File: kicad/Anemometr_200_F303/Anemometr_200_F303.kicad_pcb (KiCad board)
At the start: 2 copper layers, 25.8 x 45.3 mm, 44 parts, among them J1 Conn_01x01_Female, J10 USB_B_Micro, J11 Conn_01x01_Female, J12 Conn_01x01_Female, J13 Conn_01x01_Female, J14 Conn_01x01_Female, J15 Conn_01x01_Female, J16 Conn_01x01_Female, J17 Conn_01x01_Female, J18 Conn_01x01_Female, J19 Conn_01x01_Female, J2 Conn_01x01_Female, J20 Conn_01x01_Female, J21 Conn_01x01_Female, J22 Conn_01x01_Female, J23 Conn_01x01_Female, J24 Conn_01x01_Female, J25 Conn_01x01_Female, J26 Conn_01x01_Female, J27 Conn_01x01_Female, J3 Conn_01x01_Female, J4 Conn_01x01_Female, J5 Conn_01x01_Female, J6 Conn_01x01_Female, U1 AP1117-33, U2 STM32F303CCTx, U3 CH340C, Y1 16MHz

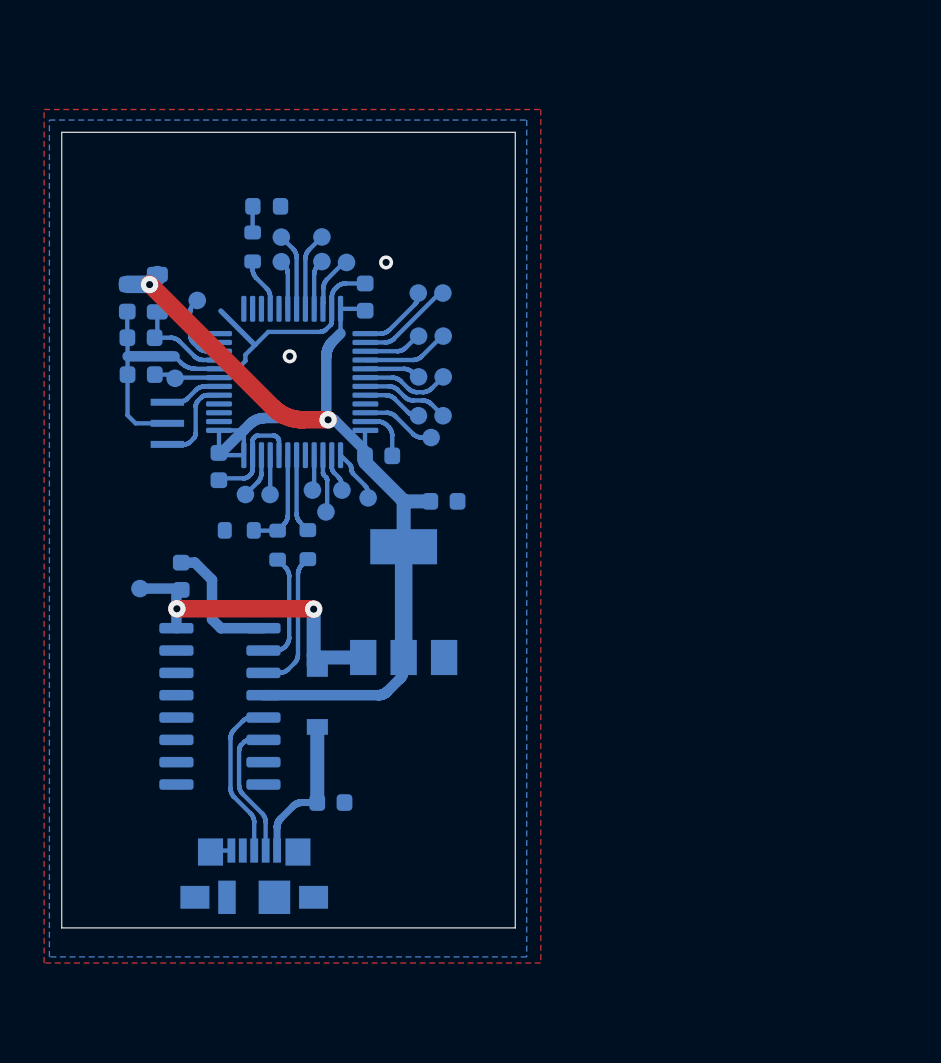
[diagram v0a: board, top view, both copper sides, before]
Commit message: изменено:      Documents/matLab/convData.m 	изменено:      kicad/Anemometr_200_F303/Anemometr_200_F303-cache.lib 	изменено:      kicad/Anemometr_200_F303/Anemometr_200_F303.kicad_pcb 	изменено:      kicad/Anemometr_200_F303/Anemometr_200_F303.kicad_pcb-bak 	изменено:      kicad/Anemometr_200_F303/Anemometr_200_F303.sch 	изменено:      kicad/Anemometr_200_F303/Anemometr_200_F303.sch-bak 	изменено:      kicad/Anemometr_200_F303/fp-info-cache 	изменено:      stm32cubeide/Anemometer_200_F303/Anemometer_200_F303.ioc 	новый файл:    stm32cubeide/Anemometer_200_F303/Core/Inc/FFTImplementationCallback.h 	изменено:      stm32cubeide/Anemometer_200_F303/Core/Inc/main.h 	новый файл:    stm32cubeide/Anemometer_200_F303/Core/Inc/maxEnvHilbert.h 	новый файл:    stm32cubeide/Anemometer_200_F303/Core/Inc/maxEnvHilbert_data.h 	новый файл:    stm32cubeide/Anemometer_200_F303/Core/Inc/maxEnvHilbert_terminate.h 	новый файл:    stm32cubeide/Anemometer_200_F303/Core/Inc/rt_nonfinite.h 	новый файл:    stm32cubeide/Anemometer_200_F303/Core/Inc/rtwtypes.h 	новый файл:    stm32cubeide/Anemometer_200_F303/Core/Inc/tmwtypes.h 	новый файл:    stm32cubeide/Anemometer_200_F303/Core/Src/FFTImplementationCallback.c 	изменено:      stm32cubeide/Anemometer_200_F303/Core/Src/main.c 	новый файл:    stm32cubeide/Anemometer_200_F303/Core/Src/maxEnvHilbert.c 	новый файл:    stm32cubeide/Anemometer_200_F303/Core/Src/maxEnvHilbert_data.c 	новый файл:    stm32cubeide/Anemometer_200_F303/Core/Src/maxEnvHilbert_terminate.c 	новый файл:    stm32cubeide/Anemometer_200_F303/Core/Src/rt_nonfinite.c 	изменено:      stm32cubeide/Anemometer_200_F303/Core/Src/stm32f3xx_hal_msp.c 	изменено:      stm32cubeide/Anemometer_200_F303/Core/Src/stm32f3xx_it.c 	изменено:      stm32cubeide/Anemometer_200_F303/Debug/Anemometer_200_F303.elf 	изменено:      stm32cubeide/Anemometer_200_F303/Debug/Anemometer_200_F303.list 	изменено:      stm32cubeide/Anemometer_200_F303/Debug/Anemometer_200_F303.map 	изменено:      stm32cubeide/Anemo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
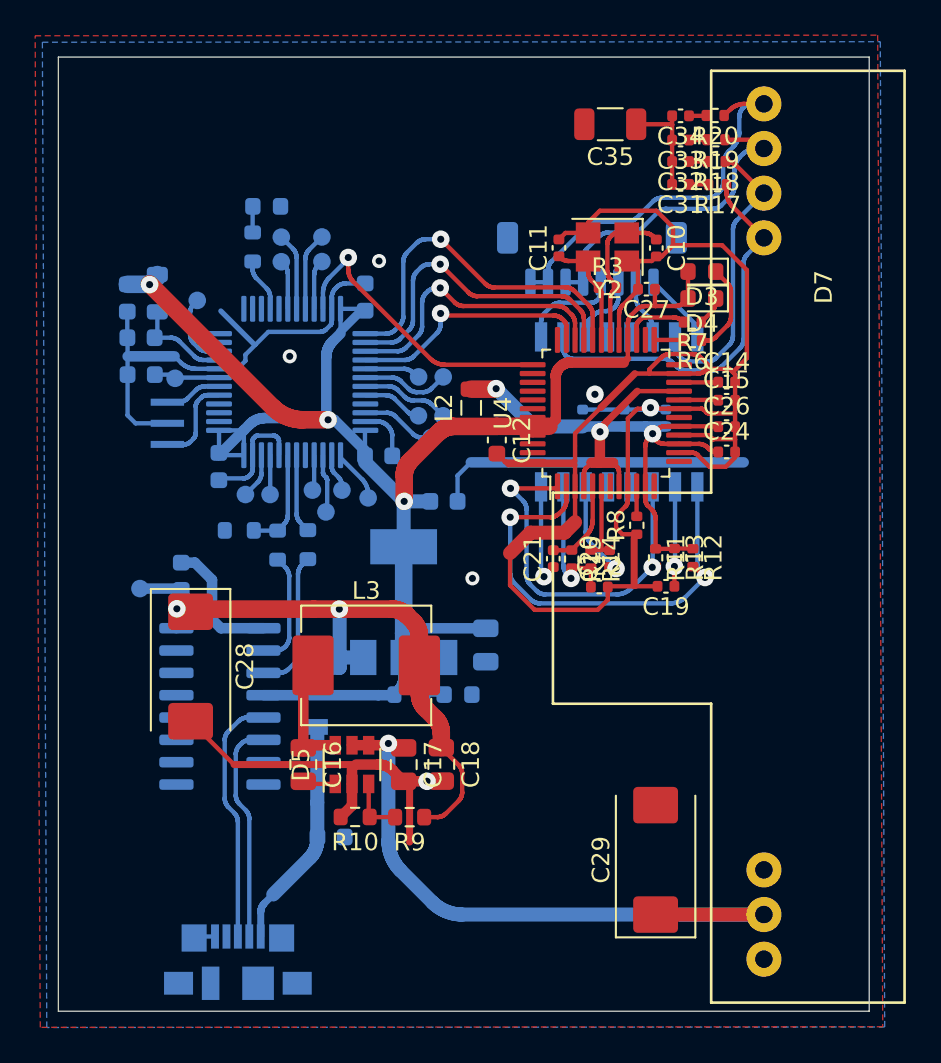
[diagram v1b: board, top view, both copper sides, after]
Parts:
- removed J18, J20, J21, J22, J24: Conn_01x01_Female, My-library:mini_conn
- added C10: C, Capacitor_SMD:C_0402_1005Metric, F.Cu at (65.3, 50.3)
- added C11: C, Capacitor_SMD:C_0402_1005Metric, F.Cu at (59.7, 50.3)
- added C12: C, Capacitor_SMD:C_0603_1608Metric, F.Cu at (56.2, 61.2)
- added C13: C, Capacitor_SMD:C_0402_1005Metric, B.Cu at (63.5, 60.0)
- added C14: 10n, Capacitor_SMD:C_0402_1005Metric, F.Cu at (69.3, 57.9)
- added C15: 4.7u, Capacitor_SMD:C_0402_1005Metric, F.Cu at (69.3, 59.0)
- added C16: 100n, Capacitor_SMD:C_0805_2012Metric, F.Cu at (45.2, 79.7)
- added C17: C, Capacitor_SMD:C_0805_2012Metric, F.Cu at (50.9, 79.7)
- added C18: C, Capacitor_SMD:C_0805_2012Metric, F.Cu at (53.0, 79.7)
- added C19: 22n, Capacitor_SMD:C_0402_1005Metric, F.Cu at (65.8, 69.5)
- added C20: 6.8n, Capacitor_SMD:C_0402_1005Metric, F.Cu at (62.6, 68.0)
- added C21: 6.8n, Capacitor_SMD:C_0402_1005Metric, F.Cu at (59.4, 68.0)
- added C22: 10n, Capacitor_SMD:C_0402_1005Metric, F.Cu at (62.0, 69.6)
- added C23: C, Capacitor_SMD:C_0402_1005Metric, B.Cu at (61.1, 60.0)
- added C24: C, Capacitor_SMD:C_0402_1005Metric, F.Cu at (69.3, 61.9)
- added C25: C, Capacitor_SMD:C_0402_1005Metric, B.Cu at (65.8, 60.0)
- added C26: C, Capacitor_SMD:C_0402_1005Metric, F.Cu at (69.3, 60.5)
- added C27: C, Capacitor_SMD:C_0402_1005Metric, F.Cu at (64.7, 52.6)
- added C28: 1000, Capacitor_Tantalum_SMD:CP_EIA-7343-15_Kemet-W, F.Cu at (38.8, 74.1)
- added C29: CP, Capacitor_Tantalum_SMD:CP_EIA-7343-15_Kemet-W, F.Cu at (65.2, 85.1)
- added C30: C, Capacitor_SMD:C_0805_2012Metric, B.Cu at (55.6, 72.9)
- added C31: 6.8n, Capacitor_SMD:C_0402_1005Metric, F.Cu at (66.7, 46.7)
- added C32: 6.8n, Capacitor_SMD:C_0402_1005Metric, F.Cu at (66.7, 45.4)
- added C33: 6.8n, Capacitor_SMD:C_0402_1005Metric, F.Cu at (66.7, 44.2)
- added C34: 6.8n, Capacitor_SMD:C_0402_1005Metric, F.Cu at (66.7, 42.8)
- added C35: 6.8n, Capacitor_SMD:C_1206_3216Metric, F.Cu at (62.7, 43.3)
- added D3: LED, LED_SMD:LED_0603_1608Metric, F.Cu at (67.9, 51.6)
- added D4: LED, LED_SMD:LED_0603_1608Metric, F.Cu at (67.9, 53.2)
- added D5: LMR50410, Package_TO_SOT_SMD:SOT-23-6, F.Cu at (48.0, 79.7)
- added D6: H1102NL, My-library:H1102N, B.Cu at (63.2, 59.6)
- added D7: RT9400, My-library:TR9400, F.Cu at (71.4, 52.2)
- added D8: LED, LED_SMD:LED_0603_1608Metric, B.Cu at (54.0, 75.7)
- added J7: Conn_01x08, Connector_JST:JST_SH_BM08B-SRSS-TB_1x08-1MP_P1.00mm_Vertical, B.Cu at (61.6, 50.9)
- added L2: L, Inductor_SMD:L_0805_2012Metric, F.Cu at (54.8, 59.4)
- added L3: 4.7u, Inductor_SMD:L_Abracon_ASPI-0630LR, F.Cu at (48.8, 74.0)
- added R10: 22.1k, Resistor_SMD:R_0603_1608Metric, F.Cu at (48.1, 82.7)
- added R11: 49R9, Resistor_SMD:R_0402_1005Metric, F.Cu at (65.2, 67.9)
- added R12: 49R9, Resistor_SMD:R_0402_1005Metric, F.Cu at (67.4, 67.9)
- added R13: 10R, Resistor_SMD:R_0402_1005Metric, F.Cu at (66.3, 67.9)
- added R14: 82R, Resistor_SMD:R_0402_1005Metric, F.Cu at (61.6, 68.0)
- added R15: 82R, Resistor_SMD:R_0402_1005Metric, F.Cu at (60.5, 68.0)
- added R16: 1k, Resistor_SMD:R_0603_1608Metric, B.Cu at (51.2, 75.7)
- added R17: 75, Resistor_SMD:R_0402_1005Metric, F.Cu at (68.8, 46.7)
- added R18: 75, Resistor_SMD:R_0402_1005Metric, F.Cu at (68.7, 45.4)
- added R19: 75, Resistor_SMD:R_0402_1005Metric, F.Cu at (68.7, 44.1)
- added R20: 75, Resistor_SMD:R_0402_1005Metric, F.Cu at (68.6, 42.8)
- added R3: 1M, Resistor_SMD:R_0402_1005Metric, F.Cu at (62.5, 52.5)
- added R6: 1M, Resistor_SMD:R_0402_1005Metric, F.Cu at (67.3, 55.6)
- added R7: 1M, Resistor_SMD:R_0402_1005Metric, F.Cu at (67.3, 54.5)
- added R8: 12.4k, Resistor_SMD:R_0402_1005Metric, F.Cu at (64.2, 66.1)
- added R9: 88.7k, Resistor_SMD:R_0603_1608Metric, F.Cu at (51.2, 82.7)
- added U4: W5500, Package_QFP:LQFP-48_7x7mm_P0.5mm, F.Cu at (62.4, 59.7)
- added Y2: Crystal_GND24_Small, Crystal:Crystal_SMD_SeikoEpson_FA238-4Pin_3.2x2.5mm, F.Cu at (62.5, 50.2)
- moved J10 4.98 mm to (41.5, 90.9)
- moved C9 1.96 mm to (46.8, 83.8)
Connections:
- net Net-(C2-Pad1) renamed +5v
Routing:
- net GND: track 46.4 -> 193.3 mm, vias 2 -> 6
- net +3.3VA: track 0.00 -> 41.4 mm, vias 0 -> 3
- net +24v: track 0.00 -> 38.2 mm, vias 0 -> 1
- net +3V3: track 64.7 -> 100.9 mm, vias 2 -> 3
- net Net-(D6-Pad1): track 0.00 -> 26.4 mm, vias 0 -> 2
- net Net-(D6-Pad10): track 0.00 -> 22.4 mm
- net Net-(D7-Pad1): track 0.00 -> 22.2 mm
- net Net-(D6-Pad3): track 0.00 -> 20.9 mm, vias 0 -> 2
- net +5v: track 19.0 -> 38.3 mm
- net Net-(D7-Pad2): track 0.00 -> 18.6 mm
- net Net-(D6-Pad15): track 0.00 -> 16.8 mm
- net /NSS: track 4.17 -> 20.5 mm, vias 0 -> 1
- net /EthRST: track 3.25 -> 17.0 mm, vias 0 -> 1
- net /MISO: track 3.38 -> 16.3 mm, vias 0 -> 1
- net /SCK: track 5.54 -> 18.4 mm, vias 0 -> 1
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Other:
- board size 25.8 x 45.3 mm -> 46.1 x 54.3 mm
